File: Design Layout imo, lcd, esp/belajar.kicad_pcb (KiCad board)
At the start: 2 copper layers, 48.5 x 78.5 mm, 3 parts, among them U1 module_mpu6050, U2 CR2013-MI2120

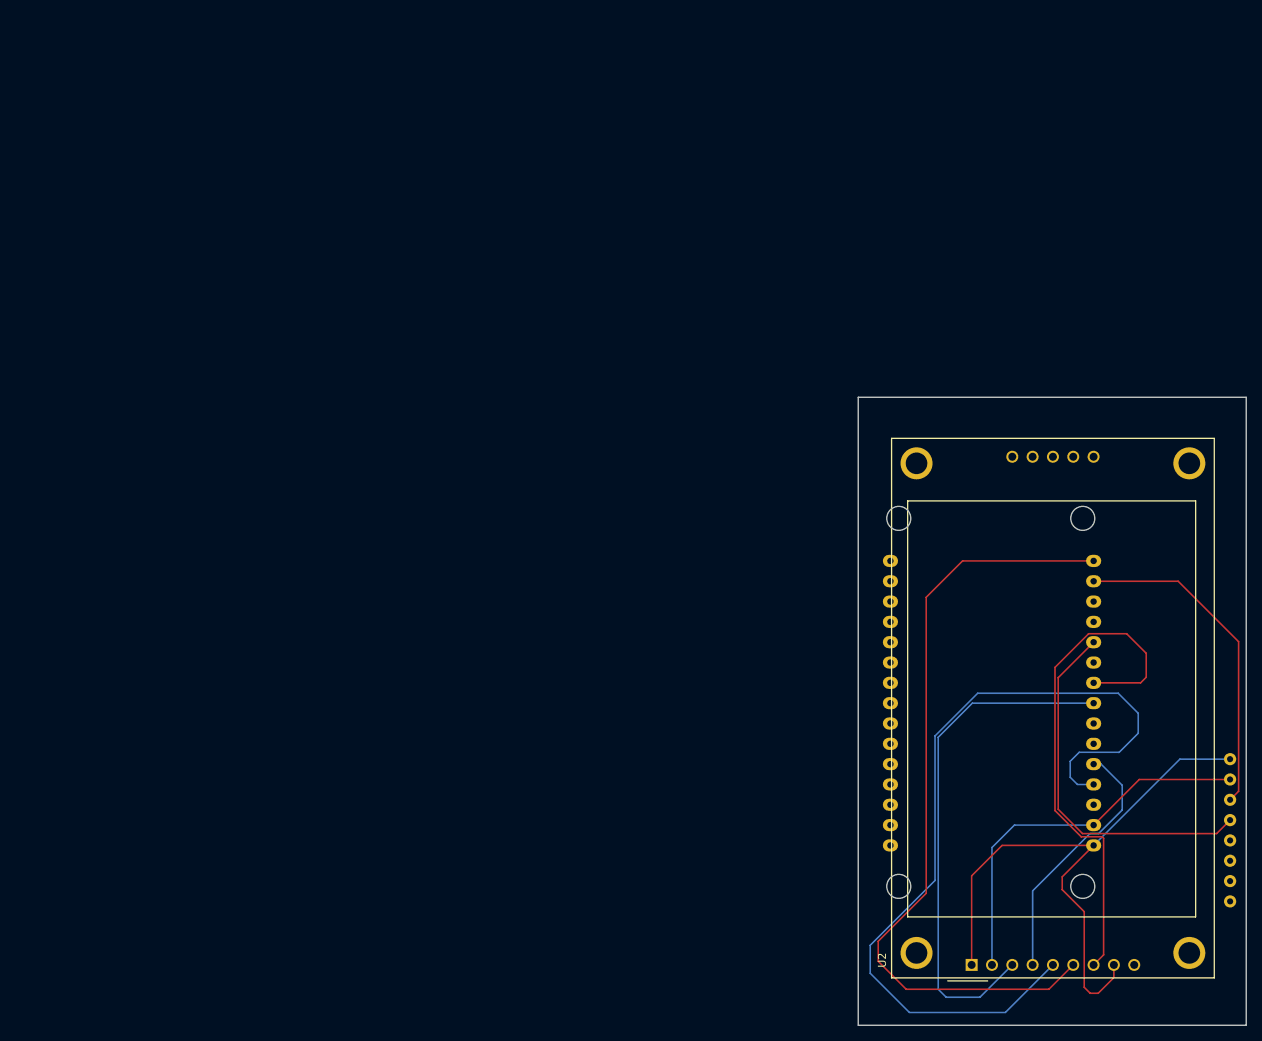
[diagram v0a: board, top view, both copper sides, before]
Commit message: test tugas awal
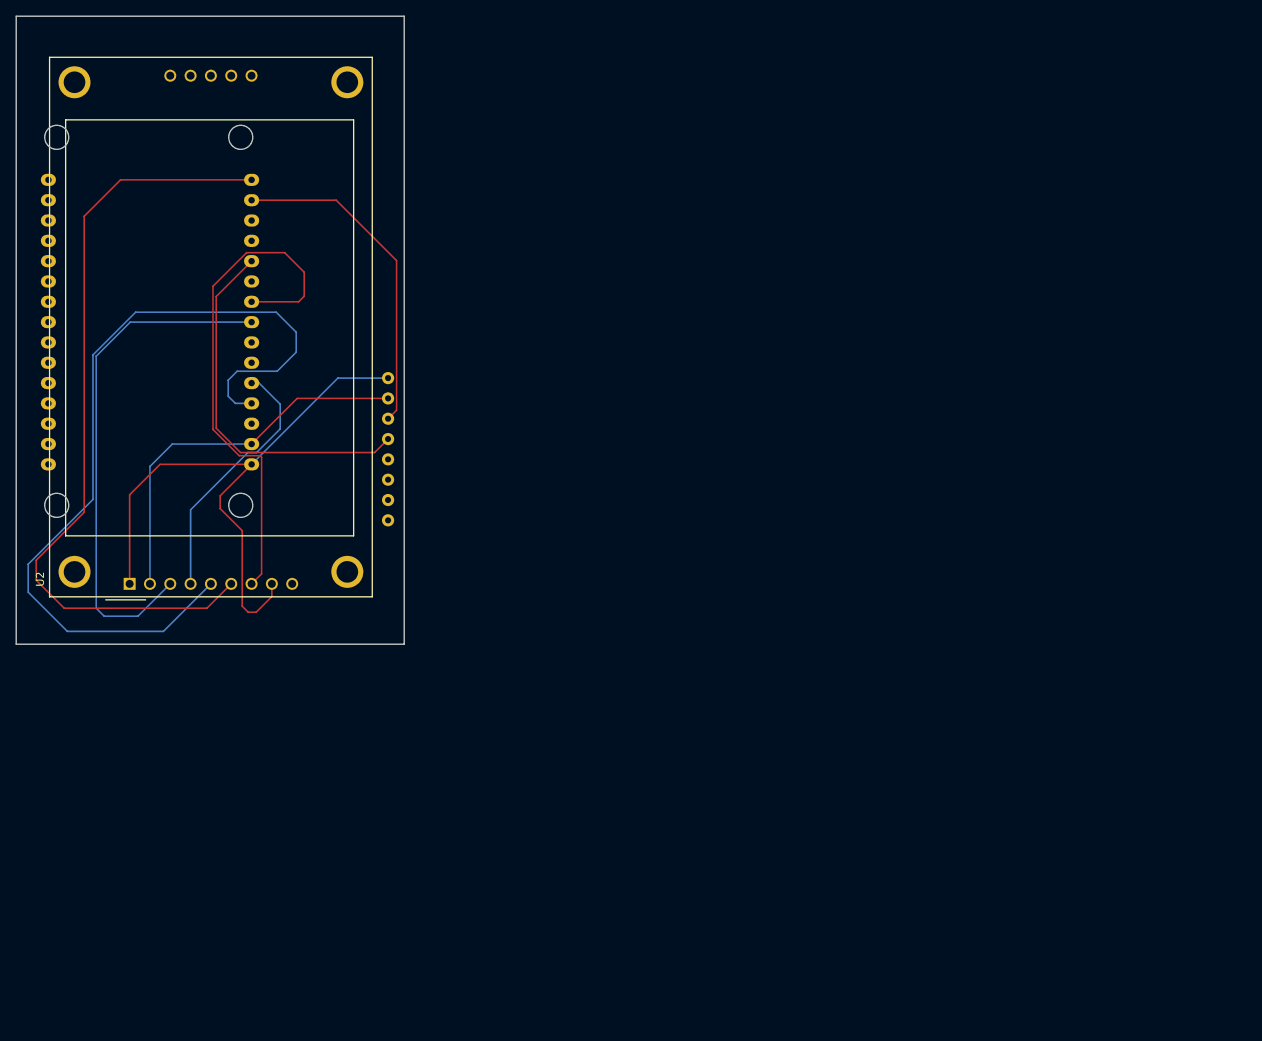
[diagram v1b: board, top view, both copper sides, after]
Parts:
- moved U2 115.5 mm to (33.0, 87.6)
- moved U4 115.5 mm to (35.3, 54.7)
- moved U1 115.5 mm to (65.3, 79.7)
